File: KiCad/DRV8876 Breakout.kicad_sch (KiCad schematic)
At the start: 12 parts, among them J1 Conn_01x08, J2 Conn_01x08, U1 DRV8876

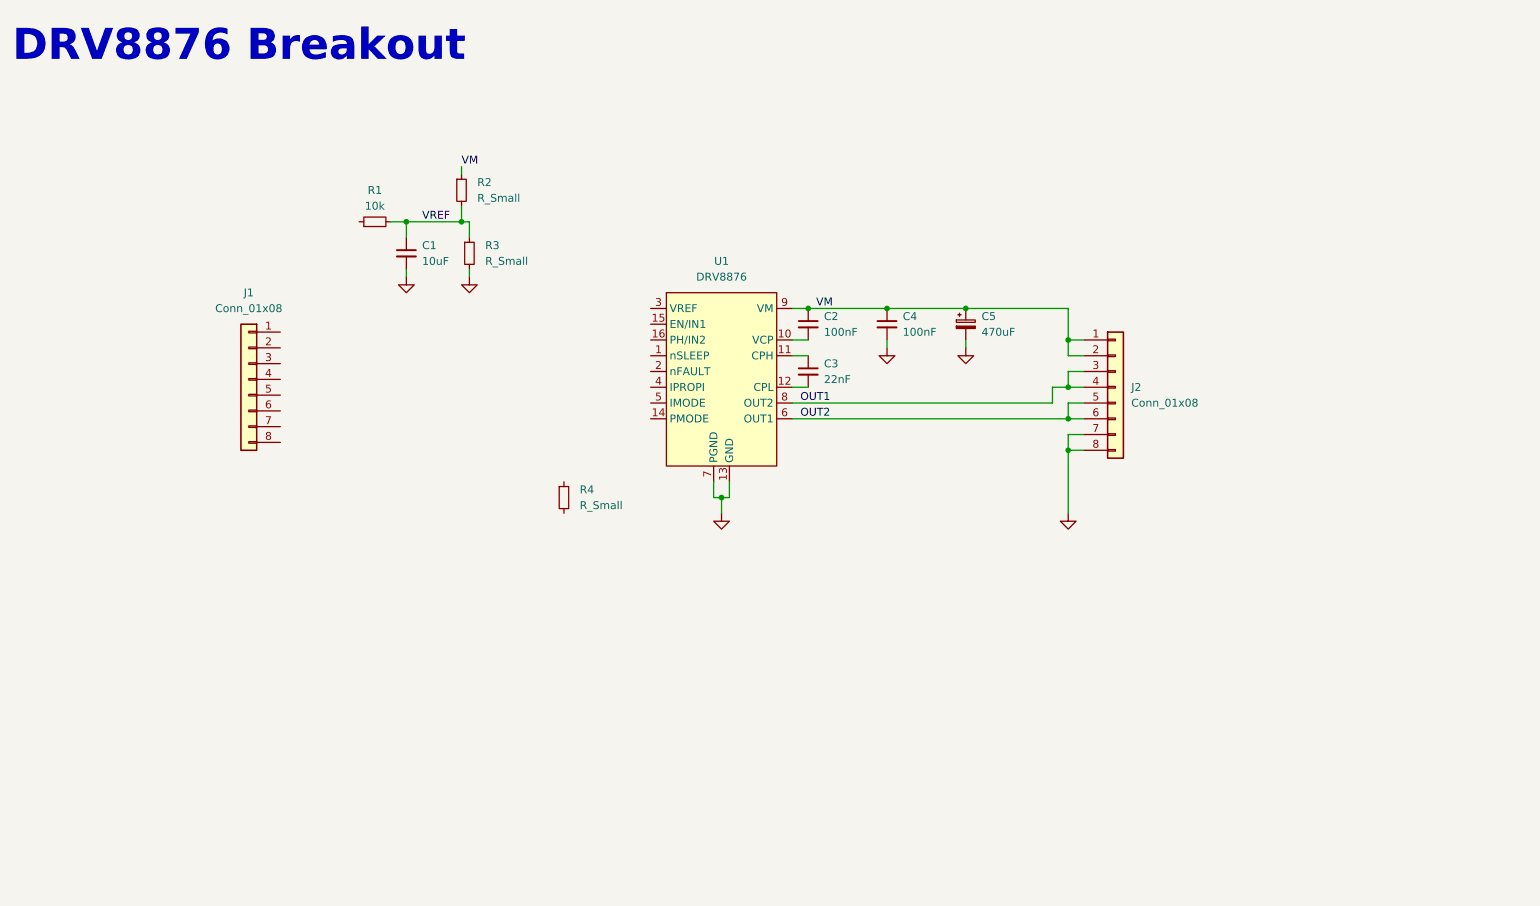
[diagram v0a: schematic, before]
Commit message: Finished Schematic and PCB
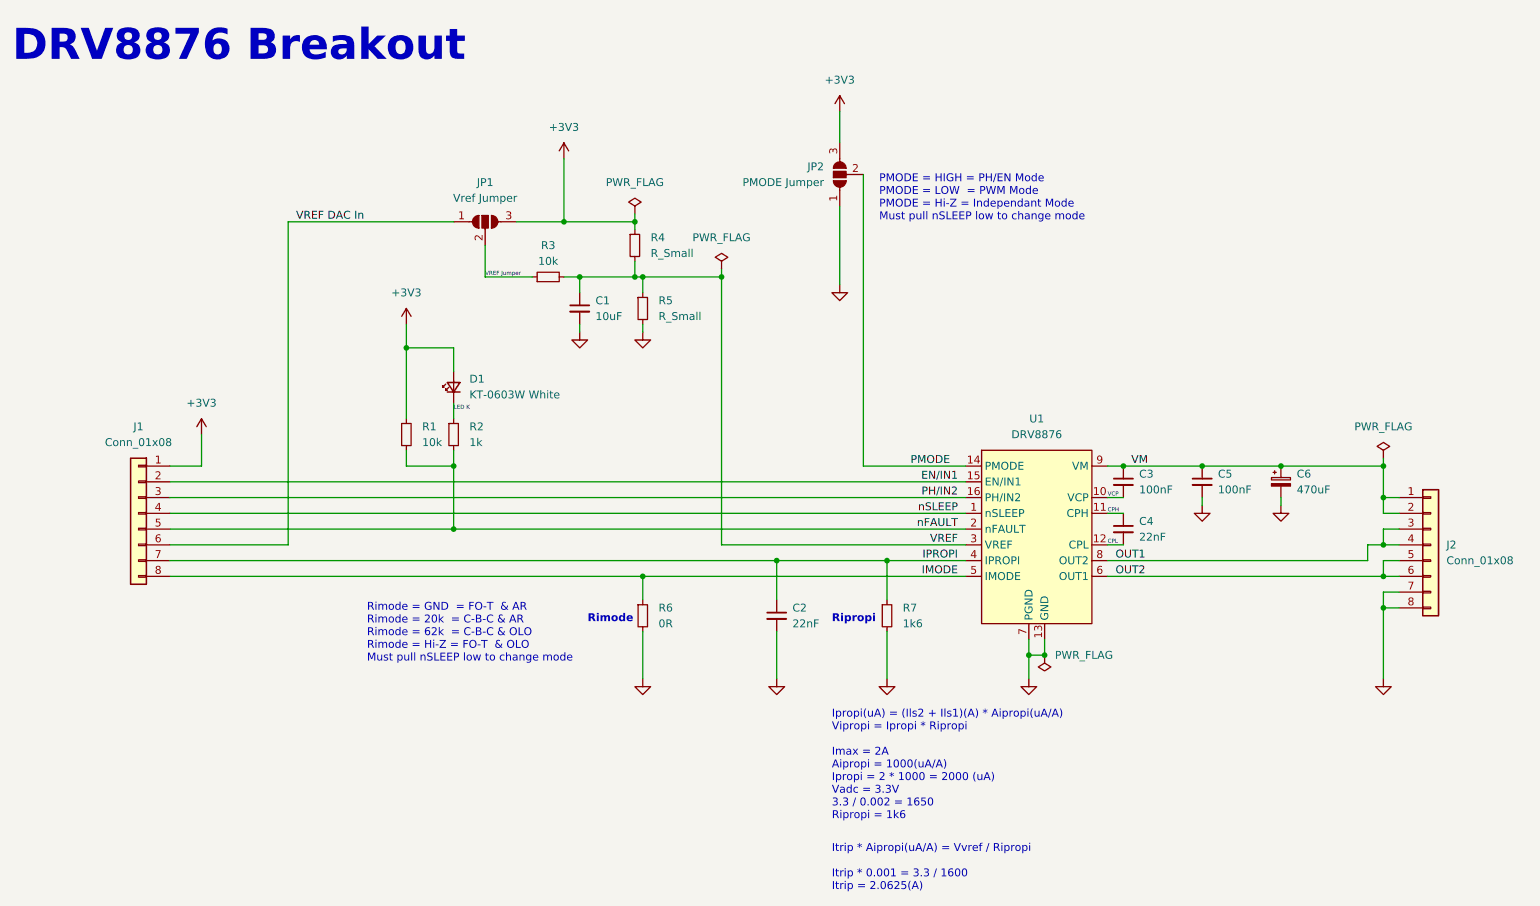
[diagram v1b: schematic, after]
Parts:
- added C2: 22nF, Capacitor_SMD:C_0603_1608Metric, symbol Device:C_Small
- added D1: KT-0603W White, LED_SMD:LED_0603_1608Metric, symbol Device:LED_Small
- added JP1: Vref Jumper, Jumper:SolderJumper-3_P2.0mm_Open_TrianglePad1.0x1.5mm_NumberLabels, symbol Jumper:SolderJumper_3_Open
- added JP2: PMODE Jumper, Jumper:SolderJumper-3_P2.0mm_Open_TrianglePad1.0x1.5mm_NumberLabels, symbol Jumper:SolderJumper_3_Open
- added R1: 10k, Resistor_SMD:R_0603_1608Metric, symbol Device:R_Small
- added R2: 1k, Resistor_SMD:R_0603_1608Metric, symbol Device:R_Small
- added R6: 0R, Resistor_SMD:R_0603_1608Metric, symbol Device:R_Small
- R7: renamed from R4; value R_Small -> 1k6
- renumbered C2 to C3, C3 to C4, C4 to C5, C5 to C6, R1 to R3, R2 to R4, R3 to R5
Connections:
- net GND: now also R7.2, C2.2, JP2.1 (A), R6.2
- net VM: no longer R4.1
- net VREF: now also U1.3 (VREF)
- net nSLEEP: now reaches U1.1 (nSLEEP)
- net nSLEEP: now also J1.4 (Pin_4)
- net VCP: now reaches C3.2, U1.10 (VCP)
- net CPH: now reaches C4.1, U1.11 (CPH)
- net CPL: now reaches C4.2, U1.12 (CPL)
- net PMODE: now reaches U1.14 (PMODE)
- net PMODE: now also JP2.2 (C)
- net EN/IN1: now reaches U1.15 (EN/IN1)
- net EN/IN1: now also J1.2 (Pin_2)
- net PH/IN2: now reaches U1.16 (PH/IN2)
- net PH/IN2: now also J1.3 (Pin_3)
- net nFAULT: now reaches U1.2 (nFAULT)
- net nFAULT: now also J1.5 (Pin_5), R1.2, R2.2
- net IPROPI: now reaches U1.4 (IPROPI)
- net IPROPI: now also J1.7 (Pin_7), R7.1, C2.1
- net IMODE: now reaches U1.5 (IMODE)
- net IMODE: now also J1.8 (Pin_8), R6.1
- net +3V3: now reaches J1.1 (Pin_1)
- net +3V3: now also R4.1, D1.2 (A), JP1.3 (B), JP2.3 (B), R1.1
- net VREF DAC In: now reaches J1.6 (Pin_6)
- net VREF DAC In: now also JP1.1 (A)
- net VREF Jumper: now reaches R3.1
- net VREF Jumper: now also JP1.2 (C)
- new net LED K: D1.1 (K), R2.1
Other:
- note added: "Ipropi(uA) = (Ils2 + Ils1)(A) * Aipropi(uA/A) Vipropi = Ipropi * Ripropi Imax = 2A Aipropi = 1000(uA/A) Ipropi = 2 * 1000 = 2000 (uA) Vadc = 3.3V 3.3 / 0.002 = 1650 Ripropi = 1k6"
- note added: "Itrip * Aipropi(uA/A) = Vvref / Ripropi Itrip * 0.001 = 3.3 / 1600 Itrip = 2.0625(A)"
- note added: "PMODE = HIGH = PH/EN Mode PMODE = LOW = PWM Mode PMODE = Hi-Z = Independant Mode Must pull nSLEEP low to change mode"
- note added: "Rimode"
- note added: "Rimode = GND = FO-T & AR Rimode = 20k = C-B-C & AR Rimode = 62k = C-B-C & OLO Rimode = Hi-Z = FO-T & OLO Must pull nSLEEP low to change mode"
- note added: "Ripropi"
- moved on the sheet: C1, C3, C4, C5, C6, J2, R3, R4, R5, R7, U1
